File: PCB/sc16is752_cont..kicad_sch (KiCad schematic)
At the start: 66 parts, among them IC13 SN74LVC1G125DBVT, IC14 LM3940IMP-3.3_NOPB, IC15 SN74LVC1G125DBVT, IC8 LMR33640ADDAR, J3 5747842-2, J4 Screw_Terminal_01x02, J5 Screw_Terminal_01x02, J6 5747842-2, Q1 SQ2319ADS-T1_BE3, Y2 ASE-14.7456MHZ-LC-T

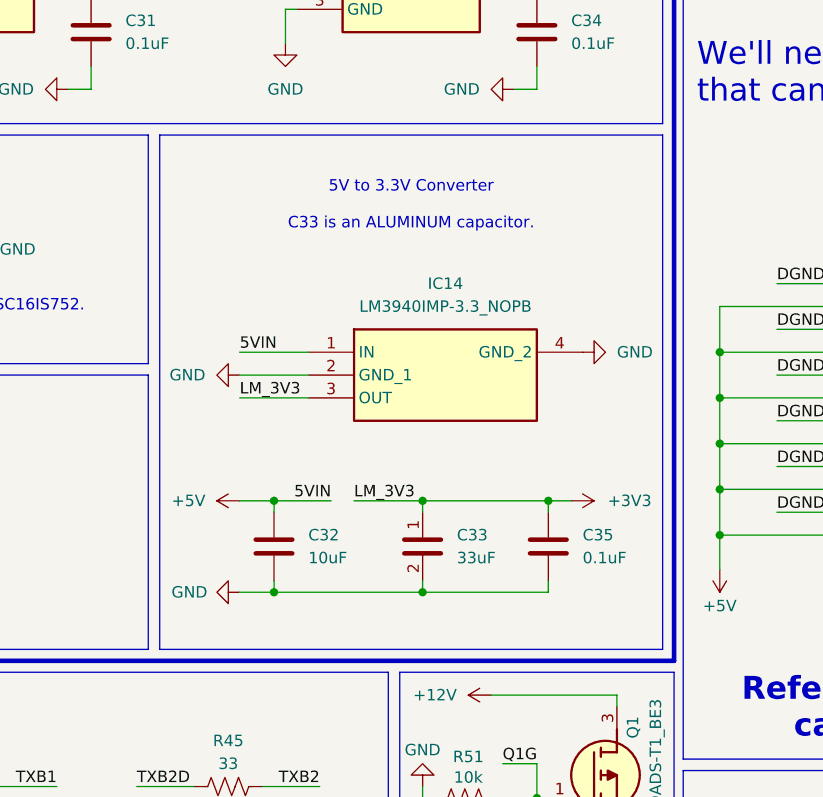
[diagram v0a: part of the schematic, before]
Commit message: Touch-ups
Various minor improvements
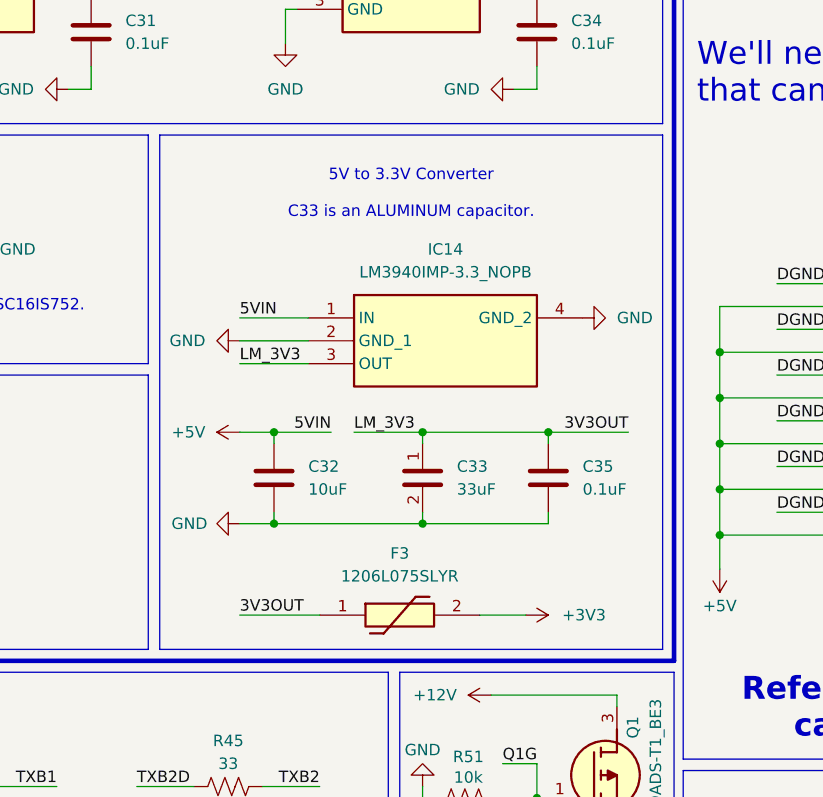
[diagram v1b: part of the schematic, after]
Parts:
- added F3: 1206L075SLYR, Fuse:Fuse_1206_3216Metric, symbol 1206L075SLYR:1206L075SLYR
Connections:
- net +3V3: now also F3.2; no longer C33.1, C35.2, IC14.3 (OUT)
- new net 3V3OUT: C33.1, C35.2, F3.1, IC14.3 (OUT)
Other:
- moved on the sheet: C32, C33, C35, IC14
